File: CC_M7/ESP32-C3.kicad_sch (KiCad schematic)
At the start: 1 part, among them U6 ESP32-C3-MINI-1-N4

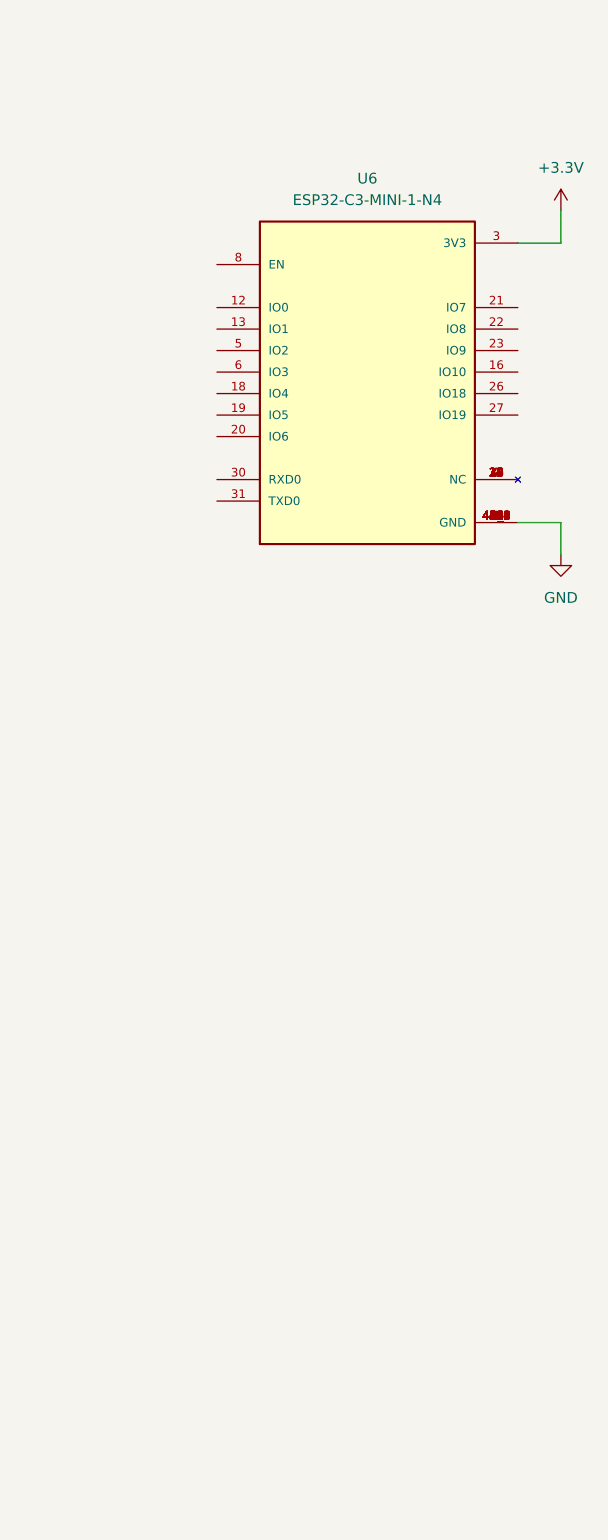
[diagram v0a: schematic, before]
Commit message: update
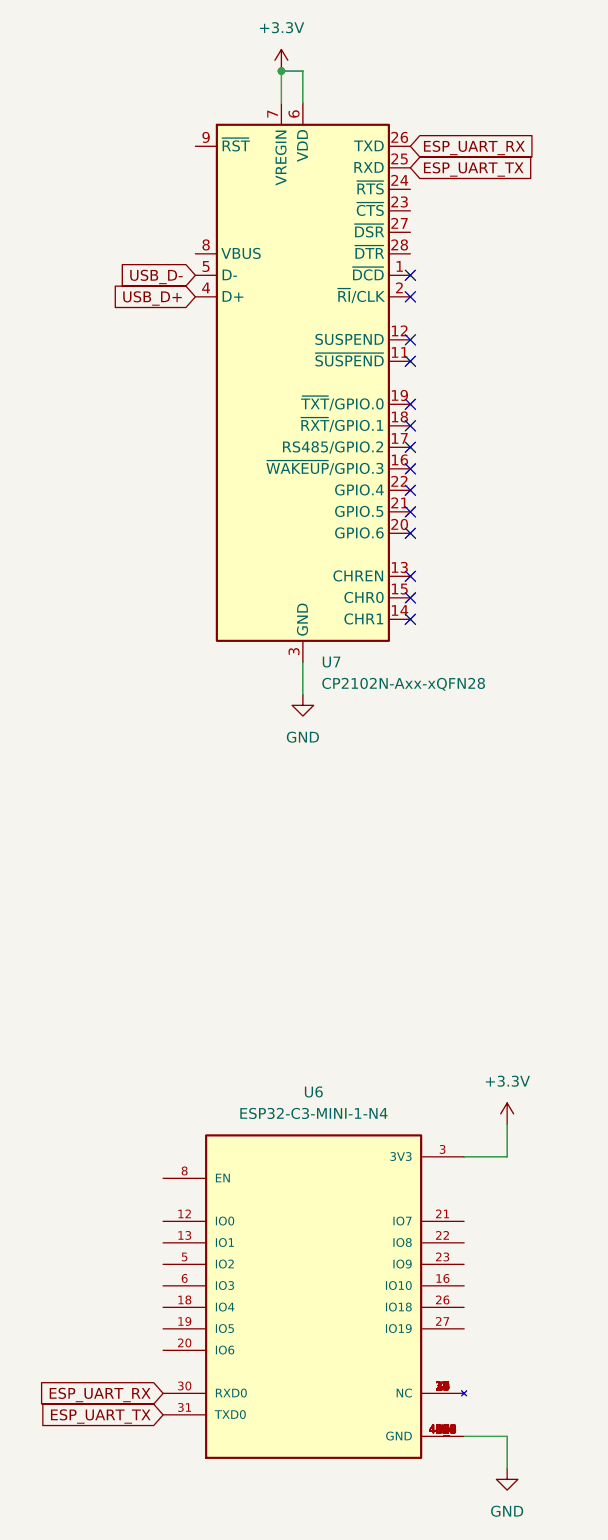
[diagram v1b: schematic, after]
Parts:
- added U7: CP2102N-Axx-xQFN28, Package_DFN_QFN:QFN-28-1EP_5x5mm_P0.5mm_EP3.35x3.35mm, symbol Interface_USB:CP2102N-Axx-xQFN28
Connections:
- net +3.3V: now also U7.6 (VDD), U7.7 (VREGIN)
- net GND: now also U7.29 (GND), U7.3 (GND)
- net ESP_UART_RX: now reaches U6.30 (RXD0)
- net ESP_UART_RX: now also U7.26 (TXD)
- net ESP_UART_TX: now reaches U6.31 (TXD0)
- net ESP_UART_TX: now also U7.25 (RXD)
- new net USB_D+: U7.4 (D+)
- new net USB_D-: U7.5 (D-)
- no-connect marks 0 -> 14
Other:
- moved on the sheet: U6
